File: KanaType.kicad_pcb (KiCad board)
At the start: 2 copper layers, 85 x 55.5 mm, 61 parts, among them J1 Conn_01x04_Socket, SW1 SW_Push, SW10 SW_Push, SW11 SW_Push, SW12 SW_Push, SW13 SW_Push, SW14 SW_Push, SW15 SW_Push, SW16 SW_Push, SW17 SW_Push, SW18 SW_Push, SW19 SW_Push, SW2 SW_Push, SW20 SW_Push, SW21 SW_Push, SW22 SW_Push, SW23 SW_Push, SW24 SW_Push, SW25 SW_Push, SW26 SW_Push, SW27 SW_Push, SW28 SW_Push, SW29 SW_Push, SW3 SW_Push, SW30 SW_Push, SW31 SW_Push, SW32 SW_Push, SW33 SW_Push, SW34 SW_Push, SW35 SW_Push, SW36 SW_Push, SW37 SW_Push, SW38 SW_Push, SW39 SW_Push, SW4 SW_Push, SW40 SW_Push, SW41 SW_Push, SW42 SW_Push, SW43 SW_Push, SW44 SW_Push, SW45 SW_Push, SW46 SW_Push, SW47 SW_Push, SW48 SW_Push, SW49 SW_Push, SW5 SW_Push, SW51 SW_Push, SW53 SW_Push, SW55 SW_Push, SW57 SW_Push, SW59 SW_Push, SW6 SW_Push, SW61 SW_Push, SW63 SW_Push, SW7 SW_Push, SW8 SW_Push, SW9 SW_Push, U1 Adafruit-Feather-RP2040

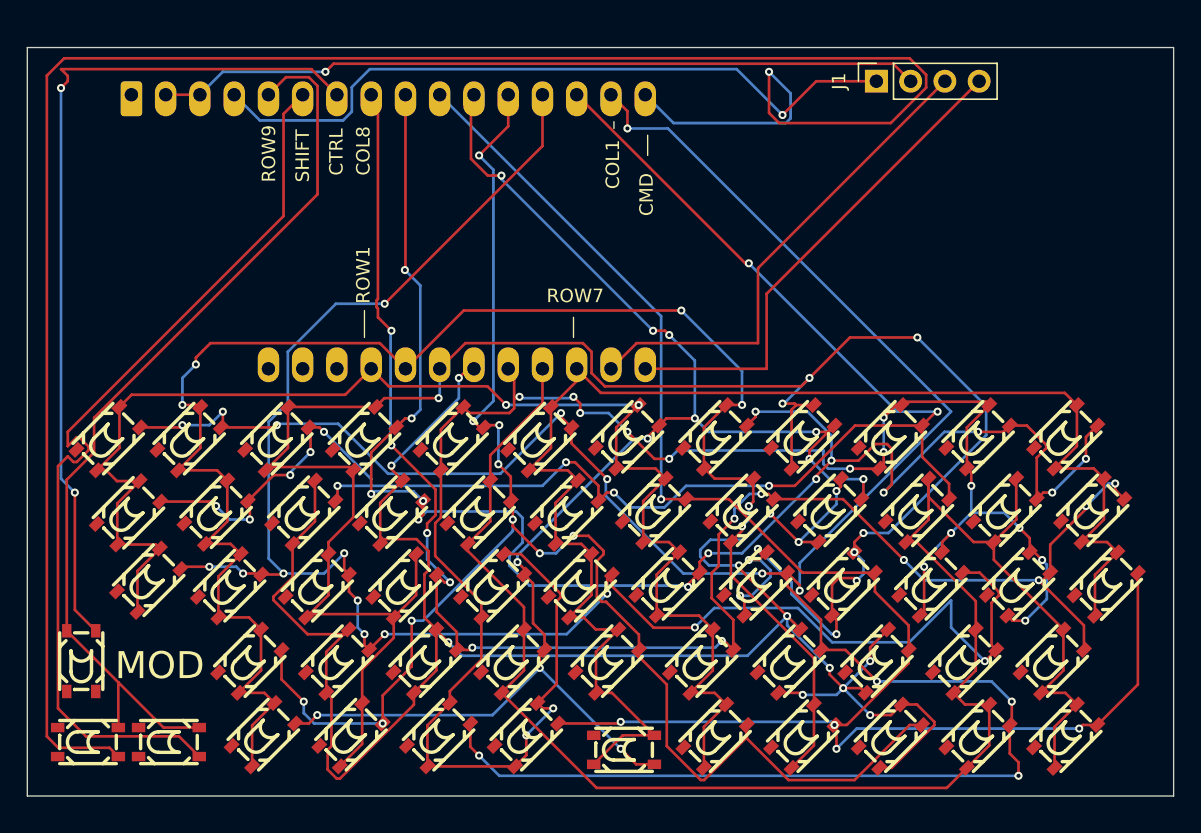
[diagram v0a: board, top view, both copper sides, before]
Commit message: Main Version
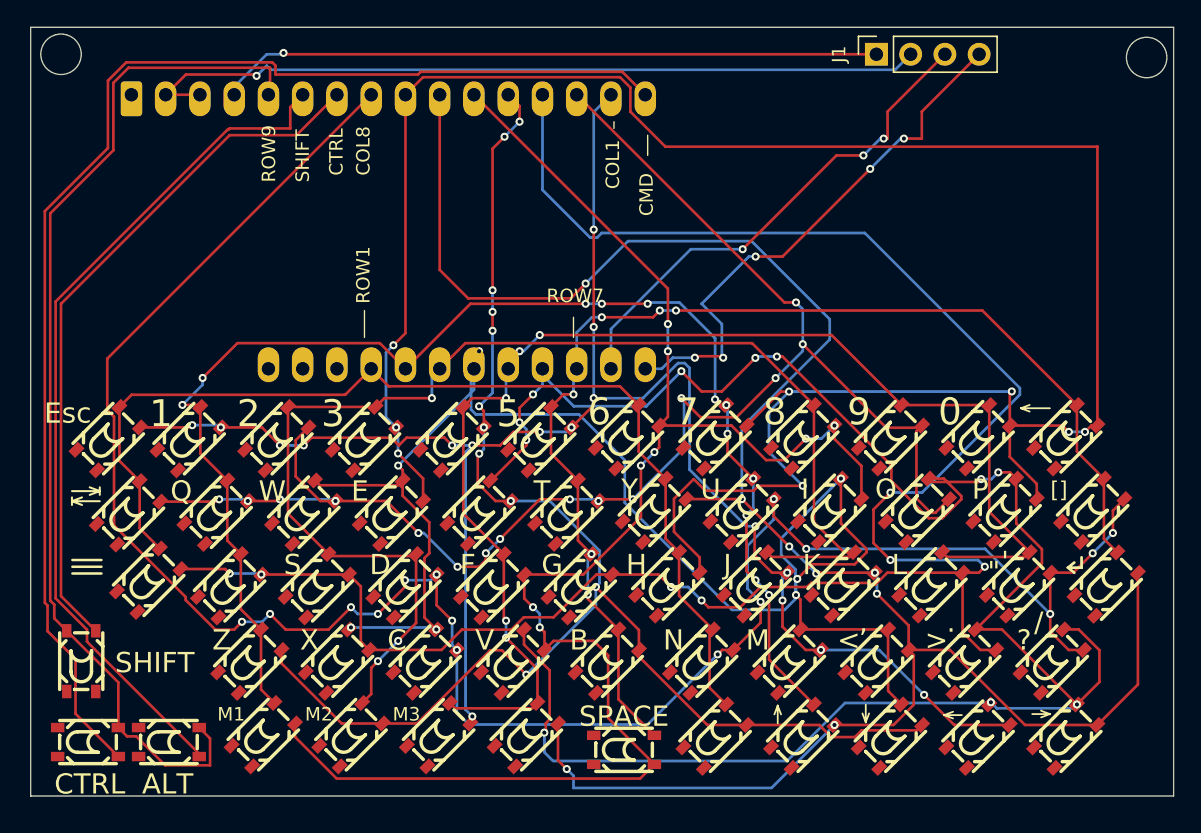
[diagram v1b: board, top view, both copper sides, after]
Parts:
- moved J1 2.00 mm to (211.0, 36.5)
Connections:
- SW1 pad 3: ROW1 -> unconnected-(SW1-Pad3)
- SW10 pad 3: ROW2 -> unconnected-(SW10-Pad3)
- SW11 pad 3: ROW2 -> unconnected-(SW11-Pad3)
- SW12 pad 3: ROW2 -> unconnected-(SW12-Pad3)
- SW13 pad 3: ROW2 -> unconnected-(SW13-Pad3)
- SW14 pad 3: ROW2 -> unconnected-(SW14-Pad3)
- SW15 pad 3: ROW2 -> unconnected-(SW15-Pad3)
- SW16 pad 3: ROW2 -> unconnected-(SW16-Pad3)
- SW17 pad 3: ROW3 -> unconnected-(SW17-Pad3)
- SW18 pad 3: ROW4 -> unconnected-(SW18-Pad3)
- SW19 pad 3: ROW3 -> unconnected-(SW19-Pad3)
- SW2 pad 3: ROW1 -> unconnected-(SW2-Pad3)
- SW20 pad 3: ROW4 -> unconnected-(SW20-Pad3)
- SW21 pad 3: ROW3 -> unconnected-(SW21-Pad3)
- SW22 pad 3: ROW4 -> unconnected-(SW22-Pad3)
- SW23 pad 3: ROW3 -> unconnected-(SW23-Pad3)
- SW24 pad 3: ROW4 -> unconnected-(SW24-Pad3)
- SW25 pad 3: ROW3 -> unconnected-(SW25-Pad3)
- SW26 pad 3: ROW4 -> unconnected-(SW26-Pad3)
- SW27 pad 3: ROW3 -> unconnected-(SW27-Pad3)
- SW28 pad 3: ROW4 -> unconnected-(SW28-Pad3)
- SW29 pad 3: ROW3 -> unconnected-(SW29-Pad3)
- SW3 pad 3: ROW1 -> unconnected-(SW3-Pad3)
- SW30 pad 3: ROW4 -> unconnected-(SW30-Pad3)
- SW31 pad 3: ROW3 -> unconnected-(SW31-Pad3)
- SW32 pad 3: ROW4 -> unconnected-(SW32-Pad3)
- SW33 pad 3: ROW5 -> unconnected-(SW33-Pad3)
- SW34 pad 3: ROW6 -> unconnected-(SW34-Pad3)
- SW35 pad 3: ROW5 -> unconnected-(SW35-Pad3)
- SW36 pad 3: ROW6 -> unconnected-(SW36-Pad3)
- SW37 pad 3: ROW5 -> unconnected-(SW37-Pad3)
- SW38 pad 3: ROW6 -> unconnected-(SW38-Pad3)
- SW39 pad 3: ROW5 -> unconnected-(SW39-Pad3)
- SW4 pad 3: ROW1 -> unconnected-(SW4-Pad3)
- SW40 pad 3: ROW6 -> unconnected-(SW40-Pad3)
- SW41 pad 3: ROW5 -> unconnected-(SW41-Pad3)
- SW42 pad 3: ROW6 -> unconnected-(SW42-Pad3)
- SW43 pad 3: ROW5 -> unconnected-(SW43-Pad3)
- SW44 pad 3: ROW6 -> unconnected-(SW44-Pad3)
- SW45 pad 3: ROW5 -> unconnected-(SW45-Pad3)
- SW46 pad 3: ROW6 -> unconnected-(SW46-Pad3)
- SW47 pad 3: ROW5 -> unconnected-(SW47-Pad3)
- SW48 pad 3: ROW6 -> unconnected-(SW48-Pad3)
- SW49 pad 3: ROW7 -> unconnected-(SW49-Pad3)
- SW5 pad 3: ROW1 -> unconnected-(SW5-Pad3)
- SW51 pad 3: ROW7 -> unconnected-(SW51-Pad3)
- SW53 pad 3: ROW7 -> unconnected-(SW53-Pad3)
- SW55 pad 3: ROW7 -> unconnected-(SW55-Pad3)
- SW57 pad 3: ROW7 -> unconnected-(SW57-Pad3)
- SW59 pad 3: ROW7 -> unconnected-(SW59-Pad3)
- SW6 pad 3: ROW1 -> unconnected-(SW6-Pad3)
- SW61 pad 3: ROW7 -> unconnected-(SW61-Pad3)
- SW63 pad 3: ROW7 -> unconnected-(SW63-Pad3)
- SW7 pad 3: ROW1 -> unconnected-(SW7-Pad3)
- SW8 pad 3: ROW1 -> unconnected-(SW8-Pad3)
- SW9 pad 3: ROW2 -> unconnected-(SW9-Pad3)
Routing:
- net ROW3: track 162.7 -> 94.7 mm, vias 11 -> 3
- net CMD: track 154.1 -> 96.3 mm, vias 1 -> 0
- net COL1: track 187.0 -> 132.8 mm, vias 12 -> 17
- net ROW5: track 142.4 -> 94.8 mm, vias 16 -> 5
- net COL7: track 123.7 -> 169.6 mm, vias 14 -> 8
- net ROW4: track 159.6 -> 114.8 mm, vias 13 -> 7
- net COL8: track 123.2 -> 159.0 mm, vias 12 -> 15
- net ROW1: track 105.2 -> 77.6 mm, vias 2 -> 0
- net ROW2: track 129.5 -> 102.1 mm, vias 6 -> 12
- net COL6: track 125.1 -> 152.1 mm, vias 5 -> 8
- net ROW7: track 108.5 -> 87.3 mm, vias 0 -> 6
- net COL3: track 133.4 -> 151.8 mm, vias 11 -> 7
- net ROW6: track 130.4 -> 146.0 mm, vias 0 -> 11
- net CTRL: track 64.4 -> 52.2 mm, vias 2 -> 0
- net COL4: track 119.2 -> 107.6 mm, vias 10 -> 11
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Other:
- board size 85 x 55.5 mm -> 84.8 x 57 mm
- board text added: "'"
- board text added: ","
- board text added: "."
- board text added: "/"
- board text added: "0"
- board text added: "1"
- board text added: "2"
- board text added: "3"
- board text added: "5"
- board text added: "6"
- board text added: "7"
- board text added: "8"
- board text added: "9"
- board text added: "<"
- board text added: ">"
- board text added: "?"
- board text added: "ALT"
- board text added: "B"
- board text added: "C"
- board text added: "D"
- board text added: "E"
- board text added: "Esc"
- board text added: "F"
- board text added: "G"
- board text added: "H"
- board text added: "I"
- board text added: "J"
- board text added: "K"
- board text added: "L"
- board text added: "M"
- board text added: "M1"
- board text added: "M2"
- board text added: "M3"
- board text added: "N"
- board text added: "O"
- board text added: "P"
- board text added: "Q"
- board text added: "S"
- board text added: "SPACE"
- board text added: "T"
- board text added: "U"
- board text added: "V"
- board text added: "W"
- board text added: "X"
- board text added: "Y"
- board text added: "Z"
- board text added: "[]"
- board text added: "{dblquote}"
- board text removed: "MOD"
- board text removed: "Powered by RP2040"
